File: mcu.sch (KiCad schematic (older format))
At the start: 22 parts, among them Q6 MMBT5551, U3 STM32F103RCTx

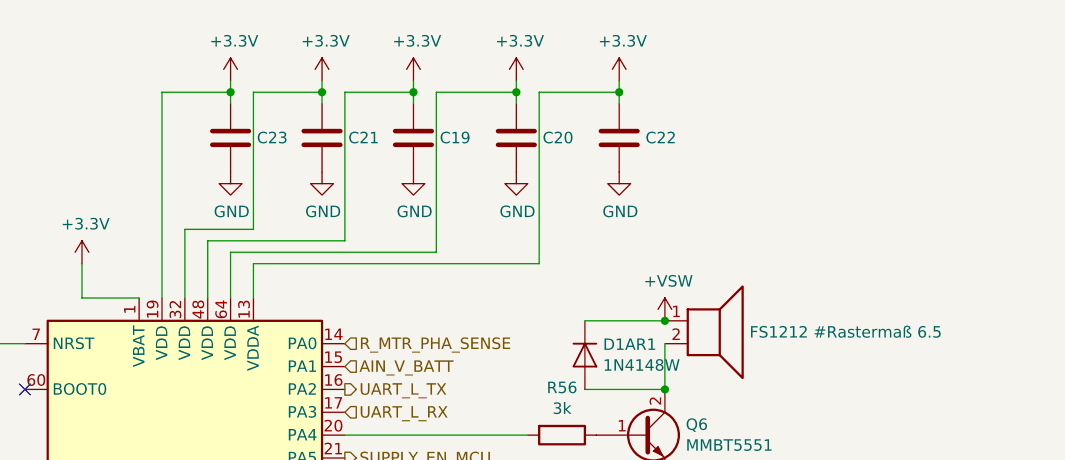
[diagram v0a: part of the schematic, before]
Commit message: Do MCU bypassing according to datasheet; annotate
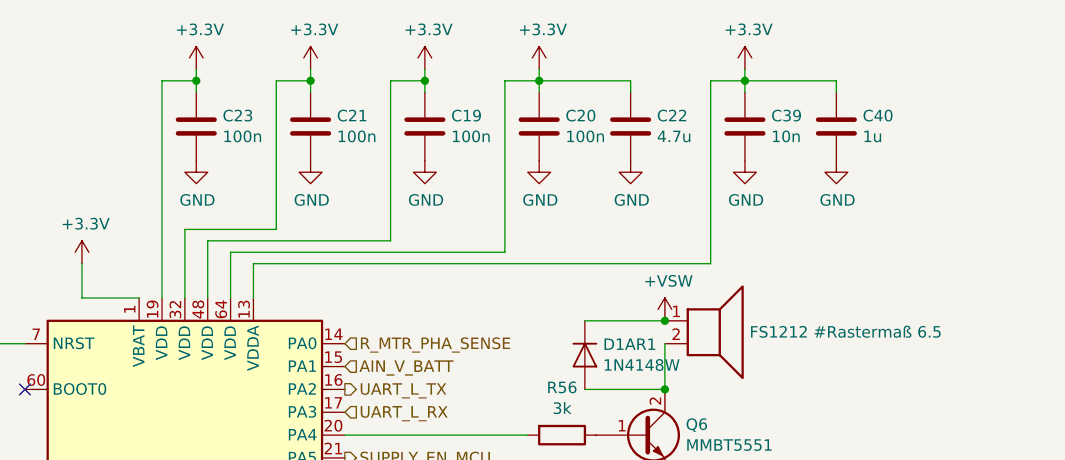
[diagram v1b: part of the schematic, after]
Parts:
- added C39: 10n, symbol Device:C
- added C40: 1u, symbol Device:C
- C19, C20, C21, C23: footprint Capacitor_SMD:C_0603_1608Metric -> (none)
- C22: value 100n -> 4.7u; footprint Capacitor_SMD:C_0603_1608Metric -> (none)
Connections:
- net +3V3: now also C39.1, C40.1
- net GND: now also C39.2, C40.2

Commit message: added footprints, continue layout
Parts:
- C19, C20, C21, C23, C39: footprint (none) -> Capacitor_SMD:C_0603_1608Metric
- C22, C40: footprint (none) -> Capacitor_SMD:C_0805_2012Metric
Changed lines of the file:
@@
 F 0 "C23" H 5815 1396 50  0000 L CNN
 F 1 "100n" H 5815 1305 50  0000 L CNN
-F 2 "" H 5738 1200 50  0001 C CNN
+F 2 "Capacitor_SMD:C_0603_1608Metric" H 5738 1200 50  0001 C CNN
 F 3 "~" H 5700 1350 50  0001 C CNN
 	1    5700 1350
@@
 F 0 "C21" H 6315 1396 50  0000 L CNN
 F 1 "100n" H 6315 1305 50  0000 L CNN
-F 2 "" H 6238 1200 50  0001 C CNN
+F 2 "Capacitor_SMD:C_0603_1608Metric" H 6238 1200 50  0001 C CNN
 F 3 "~" H 6200 1350 50  0001 C CNN
 	1    6200 1350
@@
 F 0 "C19" H 6815 1396 50  0000 L CNN
 F 1 "100n" H 6815 1305 50  0000 L CNN
-F 2 "" H 6738 1200 50  0001 C CNN
+F 2 "Capacitor_SMD:C_0603_1608Metric" H 6738 1200 50  0001 C CNN
 F 3 "~" H 6700 1350 50  0001 C CNN
 	1    6700 1350
@@
 F 0 "C20" H 7315 1396 50  0000 L CNN
 F 1 "100n" H 7315 1305 50  0000 L CNN
-F 2 "" H 7238 1200 50  0001 C CNN
+F 2 "Capacitor_SMD:C_0603_1608Metric" H 7238 1200 50  0001 C CNN
 F 3 "~" H 7200 1350 50  0001 C CNN
 	1    7200 1350
@@
 F 0 "C22" H 7715 1396 50  0000 L CNN
 F 1 "4.7u" H 7715 1305 50  0000 L CNN
-F 2 "" H 7638 1200 50  0001 C CNN
+F 2 "Capacitor_SMD:C_0805_2012Metric" H 7638 1200 50  0001 C CNN
 F 3 "~" H 7600 1350 50  0001 C CNN
 	1    7600 1350
@@
 F 0 "C39" H 8215 1396 50  0000 L CNN
 F 1 "10n" H 8215 1305 50  0000 L CNN
-F 2 "" H 8138 1200 50  0001 C CNN
+F 2 "Capacitor_SMD:C_0603_1608Metric" H 8138 1200 50  0001 C CNN
 F 3 "~" H 8100 1350 50  0001 C CNN
 	1    8100 1350
@@
 F 0 "C40" H 8615 1396 50  0000 L CNN
 F 1 "1u" H 8615 1305 50  0000 L CNN
-F 2 "" H 8538 1200 50  0001 C CNN
+F 2 "Capacitor_SMD:C_0805_2012Metric" H 8538 1200 50  0001 C CNN
 F 3 "~" H 8500 1350 50  0001 C CNN
 	1    8500 1350

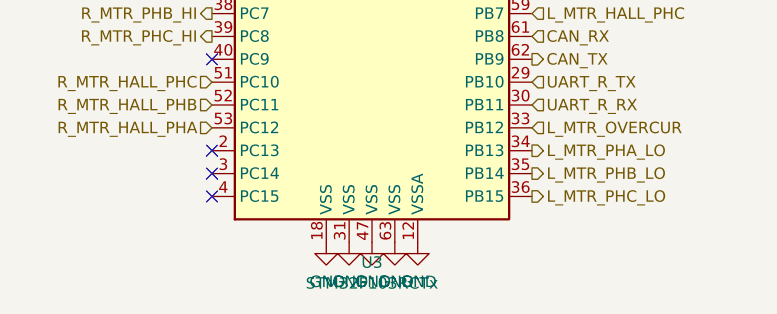
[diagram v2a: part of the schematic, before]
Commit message: add resistors on mosfet driver inputs, change board corners, fix labels
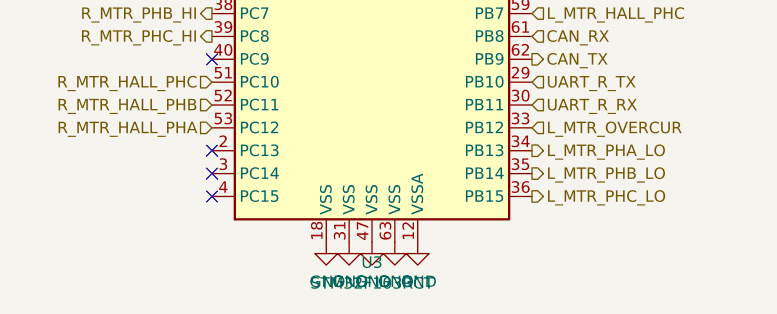
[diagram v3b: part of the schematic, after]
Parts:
- U3: value STM32F103RCTx -> STM32F103RCT
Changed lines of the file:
@@
 P 5650 3900
 F 0 "U3" H 5650 2011 50  0000 C CNN
-F 1 "STM32F103RCTx" H 5650 1920 50  0000 C CNN
+F 1 "STM32F103RCT" H 5650 1920 50  0000 C CNN
 F 2 "Package_QFP:LQFP-64_10x10mm_P0.5mm" H 5050 2200 50  0001 R CNN
 F 3 "http://www.st.com/st-web-ui/static/active/en/resource/technical/document/datasheet/CD00191185.pdf" H 5650 3900 50  0001 C CNN
